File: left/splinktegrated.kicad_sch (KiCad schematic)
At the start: 66 parts, among them J1 USB_C_Receptacle_USB2.0, J10 NA_Ribbon, J13 Conn_01x01_Socket, J14 Cirque, J15 Conn_01x01_Socket, J16 Conn_01x01_Socket, J17 Conn_01x01_Socket, J18 USB_C_Receptacle_USB2.0, J19 Conn_01x01_Socket, J20 Conn_01x01_Socket, J5 Conn_01x02, J6 Cirque, J7 NA_trackball, J8 NA_Ribbon, J9 NA_RGB, Q4 AO3401A, Q5 AO3401A, SW1 NA_SW_SPST, SW2 NA_SW_SPST, U1 RP2040, U2 USBLC6-2P6, U3 XC6210B332MR-G, U4 USBLC6-2P6, U5 W25Q128JVS, U6 74LVC1T45, Y1 Crystal_GND24

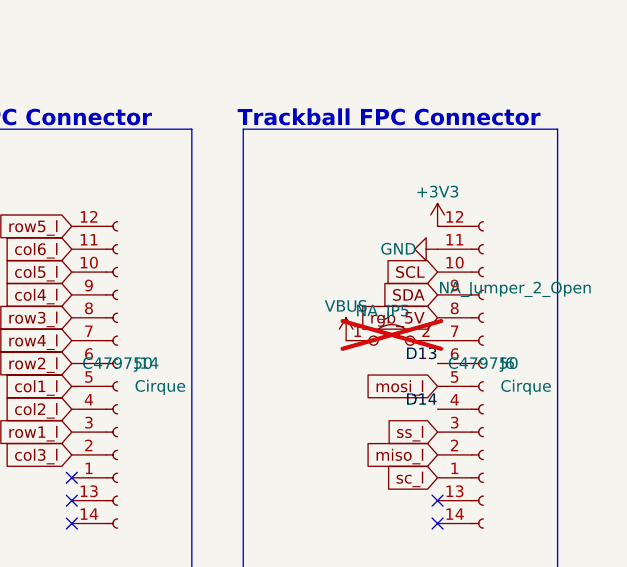
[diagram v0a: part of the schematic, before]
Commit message: routing
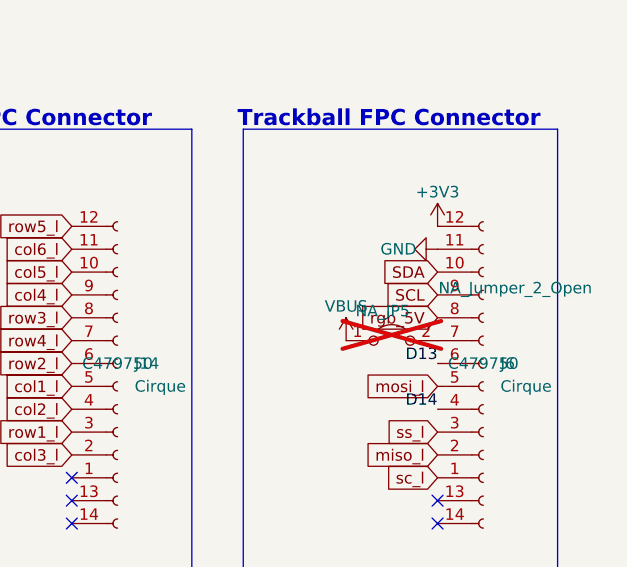
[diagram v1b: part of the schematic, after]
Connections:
- net SCL: now also J6.9 (Pin_9); no longer J6.10 (Pin_10)
- net SDA: now also J6.10 (Pin_10); no longer J6.9 (Pin_9)
